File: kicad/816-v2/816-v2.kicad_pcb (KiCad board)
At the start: 4 copper layers, 172.7 x 160 mm, 57 parts, among them J1 Barrel_Jack, J10 Mini-DIN-6, J2 UART, J3 VIA1 Port B, J4 VIA2 Connector, J5 PATA, J6 PATA_PWR, J7 Pico left, J8 Pico right, J9 DE15_Pins_HighDensity_Mountin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, SW1 SW_SPST, SW2 SW_Push, U1 W65C816SxP, U10 W65C22NxP, U11 W65C51NxP, U12 DS1813-5, U13 AS6C4008-55PCN, U2 74HC74, U3 74HC573, U4 74HC245, U5 ATF1504AS-10JU44, U6 ATtiny26L-8P, U8 SST39SF020, U9 W65C22NxP, Y1 8MHz, Y2 1.8342MHz

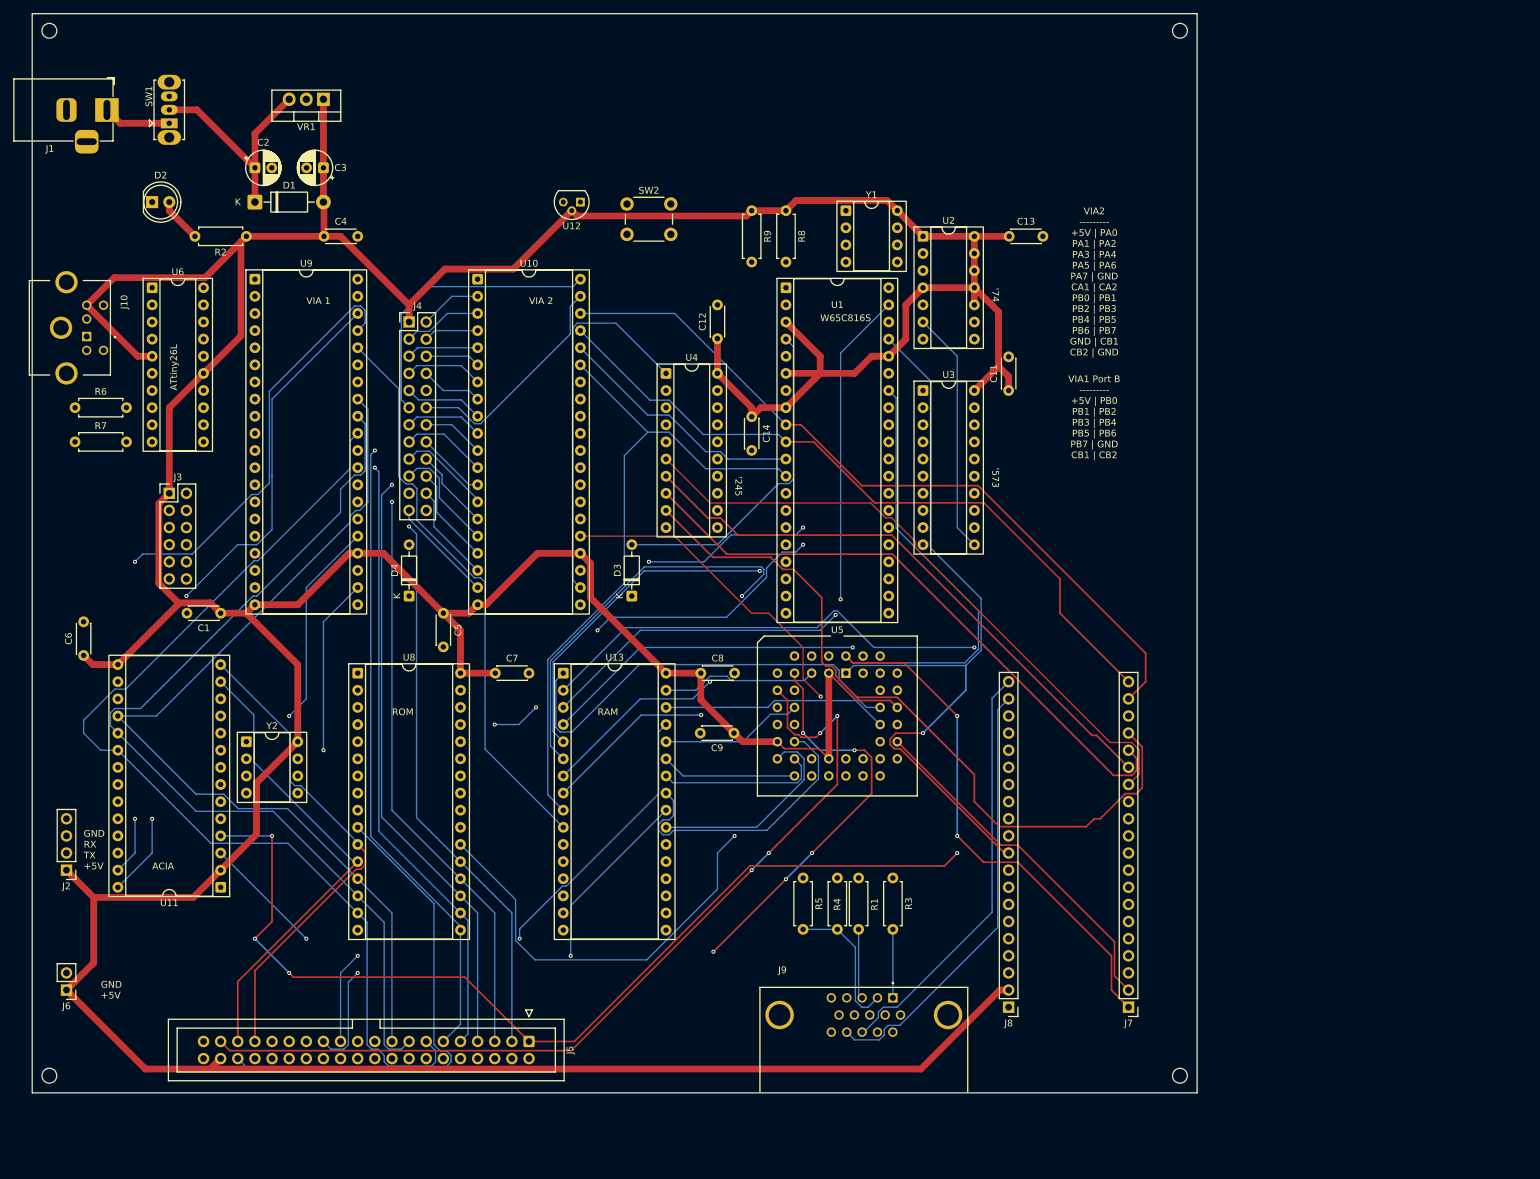
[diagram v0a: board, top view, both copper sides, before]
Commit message: Update KiCad files new pcb revision, hopefully working
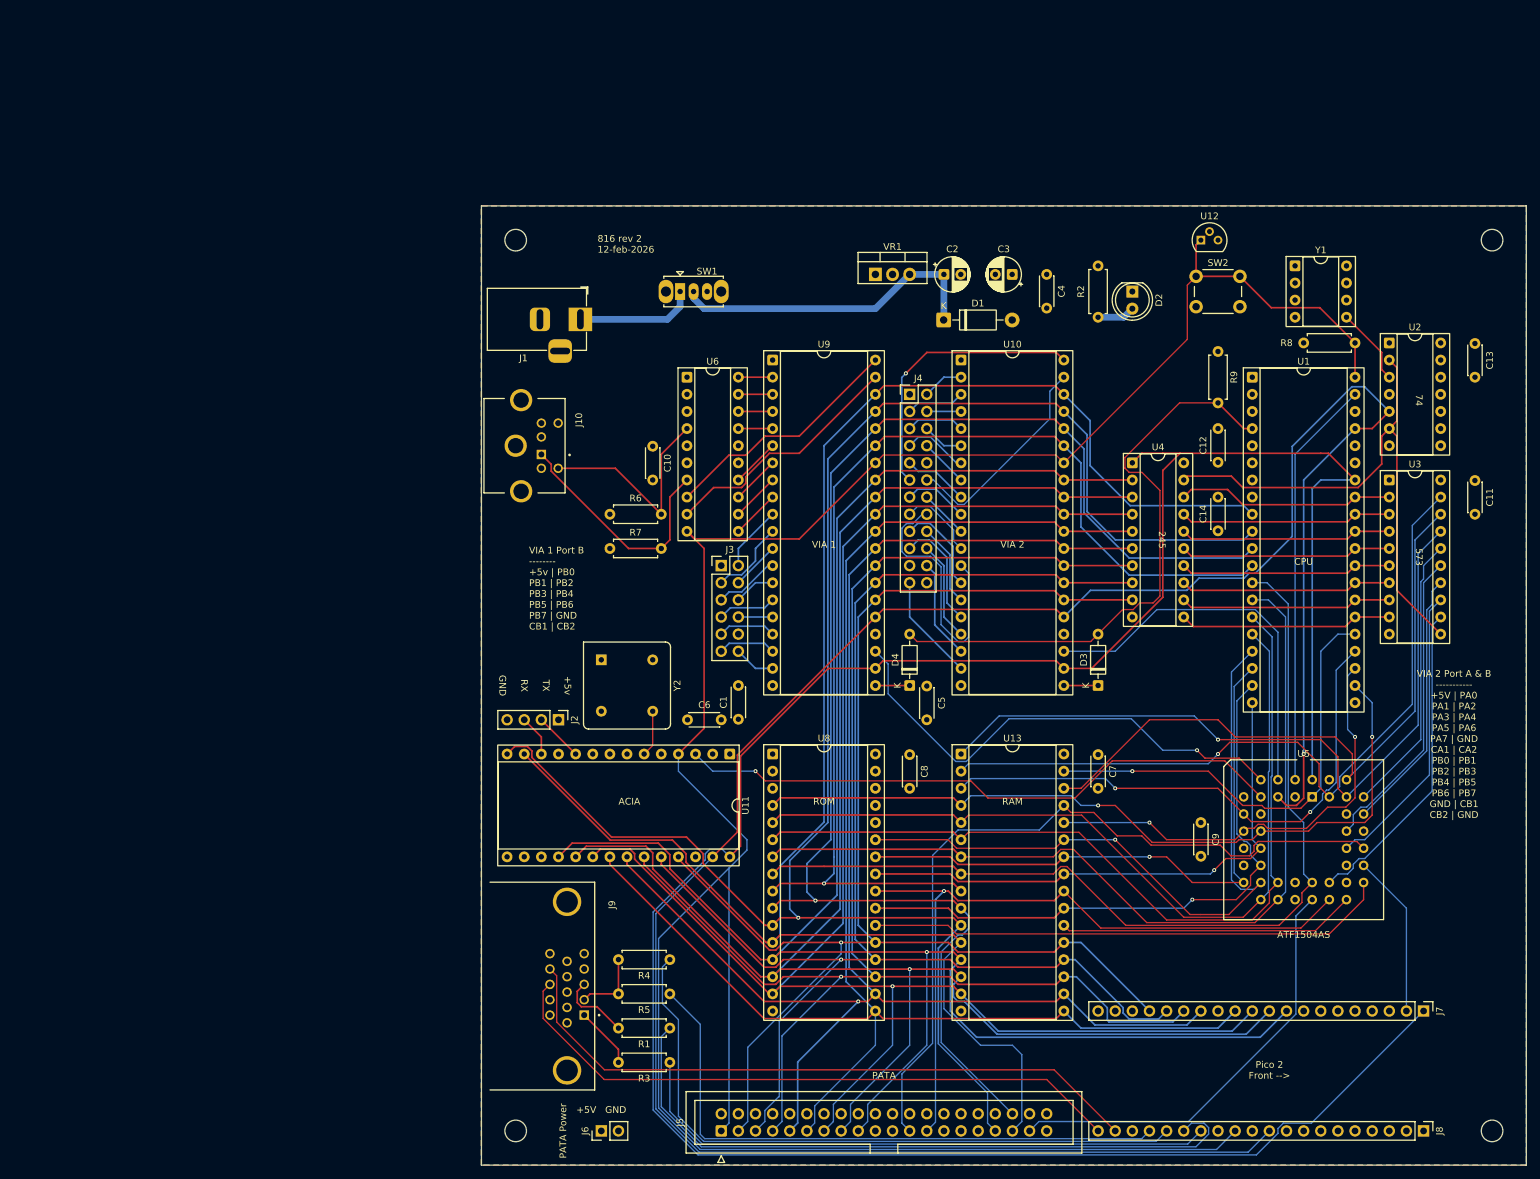
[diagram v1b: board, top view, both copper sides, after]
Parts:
- added C10: 0.1uF, Capacitor_THT:C_Disc_D4.3mm_W1.9mm_P5.00mm, F.Cu at (92.0, 56.5)
- H1, H2, H3, H4: footprint MountingHole:MountingHole_2.2mm_M2 -> MountingHole:MountingHole_3.2mm_M3
- J9: value DE15_Pins_HighDensity_MountingHoles -> DE-15 HD
- U1: value W65C816SxP -> W65C816
- U10, U9: value W65C22NxP -> W65C22S
- U11: value W65C51NxP -> W65C51
- U13: value AS6C4008-55PCN -> AS6C4008
- U5: value ATF1504AS-10JU44 -> ATF1504AS
- U6: value ATtiny26L-8P -> ATtiny26L
- VR1: value UA78L05ACPK -> 7805
- Y2: footprint Package_DIP:DIP-8_W7.62mm_Socket -> Oscillator:Oscillator_DIP-8
- moved D2 145.9 mm to (163.1, 33.6), turned to -90 degrees
- moved R2 126.4 mm to (158.0, 29.8), turned to -90 degrees
- moved C4 107.3 mm to (150.4, 31.0), turned to -90 degrees
- moved D1 103.6 mm to (135.1, 37.8)
- moved C2 103.4 mm to (135.2, 31.0)
- moved C3 103.3 mm to (145.3, 31.0)
- moved U12 92.2 mm to (173.3, 26.0), turned to 0 degrees
- moved C7 90.2 mm to (158.0, 102.2), turned to -90 degrees
- moved C6 90.0 mm to (97.2, 97.1), turned to 0 degrees
- moved VR1 85.9 mm to (125.0, 31.0), turned to 0 degrees
- moved SW2 85.1 mm to (172.6, 31.3)
- moved J3 82.5 mm to (102.2, 74.2)
- moved J6 82.0 mm to (84.4, 158.0), turned to 90 degrees
- moved R6 80.9 mm to (85.7, 66.6)
- moved R7 80.9 mm to (85.7, 71.7)
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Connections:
- C14 pad 1: VCC -> GND
- C14 pad 2: GND -> VCC
- C9 pad 1: VCC -> GND
- C9 pad 2: GND -> VCC
- J10 pad 1: Net-(J10-Pad1) -> PS2DATA
- J10 pad 5: Net-(J10-Pad5) -> PS2CLK
- J7 pad 19: A0 -> unconnected-(J7-Pin_19-Pad19)
- J7 pad 20: A1 -> unconnected-(J7-Pin_20-Pad20)
- R6 pad 1: Net-(J10-Pad5) -> VCC
- R7 pad 1: Net-(J10-Pad1) -> VCC
- U5 pad 1: PH2 -> A15
- U5 pad 11: A14 -> A13
- U5 pad 12: A13 -> A12
- U5 pad 14: A12 -> A11
- U5 pad 16: A11 -> A10
- U5 pad 17: A10 -> A9
- U5 pad 18: A8 -> A7
- U5 pad 19: A9 -> A8
- U5 pad 20: A6 -> A5
- U5 pad 21: A7 -> A6
- U5 pad 24: A4 -> IO5CS
- U5 pad 25: A5 -> A4
- U5 pad 27: WE -> A23
- U5 pad 28: ROMCS -> RAMCS
- U5 pad 29: RAMCS -> ROMCS
- U5 pad 33: A16 -> WE
- U5 pad 34: A17 -> A22
- U5 pad 36: A18 -> A20
- U5 pad 37: A19 -> A21
- U5 pad 39: A20 -> A19
- U5 pad 4: IO1CS -> IO2CS
- U5 pad 40: A22 -> A17
- U5 pad 41: A21 -> A18
- U5 pad 43: A23 -> A16
- U5 pad 5: A15 -> PH2
- U5 pad 6: IO2CS -> IO1CS
- U5 pad 9: IO5CS -> A14
- U8 pad 28: A13 -> GND
- U8 pad 29: A14 -> GND
- U8 pad 3: A15 -> GND
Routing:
- net VCC: track 778.8 -> 0.00 mm
- net D7: track 323.4 -> 208.0 mm
- net D4: track 333.3 -> 230.6 mm
- net D6: track 313.7 -> 216.5 mm
- net D3: track 338.8 -> 242.7 mm, vias 1 -> 0
- net D5: track 317.4 -> 224.4 mm
- net D2: track 327.9 -> 254.2 mm, vias 0 -> 1
- net BLUE: track 29.0 -> 102.0 mm
- net PH2: track 279.4 -> 350.9 mm, vias 4 -> 1
- net IO5CS: track 133.9 -> 64.6 mm, vias 4 -> 0
- net GREEN2: track 33.2 -> 99.2 mm
- net RED: track 22.9 -> 88.8 mm
- net A1: track 335.1 -> 269.3 mm
- net GREEN1: track 39.4 -> 90.0 mm
- net A2: track 261.4 -> 212.1 mm, vias 0 -> 1
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- added copper zone on In2.Cu, net GND
- added copper zone on B.Cu, net VCC
- added copper zone on F.Cu, net VCC
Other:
- board size 172.7 x 160 mm -> 154.9 x 142.2 mm
- board text added: "+5V GND"
- board text added: "+5v TX RX GND"
- board text added: "245"
- board text added: "573"
- board text added: "74"
- board text added: "816 rev 2 12-feb-2026"
- board text added: "ATF1504AS"
- board text added: "CPU"
- board text added: "PATA"
- board text added: "PATA Power"
- board text added: "Pico 2 Front -->"
- board text added: "VIA 1 Port B -------- +5v | PB0 PB1 | PB2 PB3 | PB4 PB5 | PB6 PB7 | GND CB1 | CB2"
- board text added: "VIA 2 Port A & B ----------- +5V | PA0 PA1 | PA2 PA3 | PA4 PA5 | PA6 PA7 | GND CA1 | CA2 PB0 | PB1 PB2 | PB3 PB4 | PB5 PB6 | PB7 GND | CB1 CB2 | GND"
- board text removed: "'245"
- board text removed: "'573"
- board text removed: "'74"
- board text removed: "ATtiny26L"
- board text removed: "GND +5V"
- board text removed: "GND RX TX +5V"
- board text removed: "VIA1 Port B --------- +5V | PB0 PB1 | PB2 PB3 | PB4 PB5 | PB6 PB7 | GND CB1 | CB2"
- board text removed: "VIA2 --------- +5V | PA0 PA1 | PA2 PA3 | PA4 PA5 | PA6 PA7 | GND CA1 | CA2 PB0 | PB1 PB2 | PB3 PB4 | PB5 PB6 | PB7 GND | CB1 CB2 | GND"
- board text removed: "W65C816S"
